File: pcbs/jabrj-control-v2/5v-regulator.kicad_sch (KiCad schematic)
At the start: 46 parts, among them Q401 DMN21D2UFB-7B, Q402 DMN21D2UFB-7B, Q403 DMN21D2UFB-7B, U401 AZV3001FZ4-7, U402 TPS259472ARPWR, U403 MAX20008AFOC/VY+T

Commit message: Layout almost done
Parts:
- D403, D404: footprint (none) -> project_footprints:C_0402
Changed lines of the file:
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@@
 			)
 		)
-		(property "Footprint" ""
+		(property "Footprint" "project_footprints:C_0402"
 			(at 228.6 109.22 90)
 			(hide yes)
@@
 			)
 		)
-		(property "Footprint" ""
+		(property "Footprint" "project_footprints:C_0402"
 			(at 254 109.22 90)
 			(hide yes)

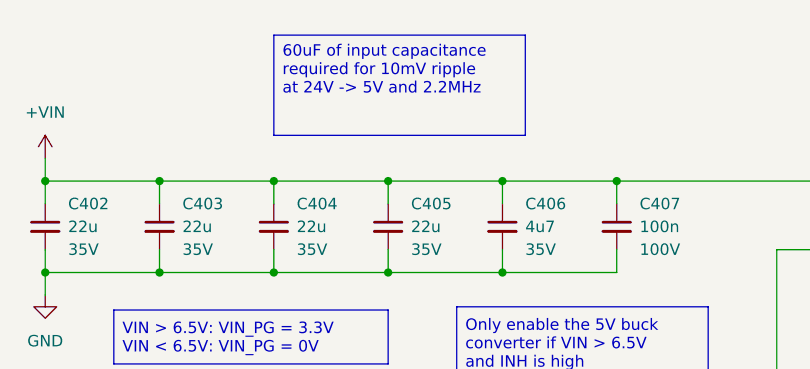
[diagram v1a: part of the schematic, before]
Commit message: 651 Unrouted
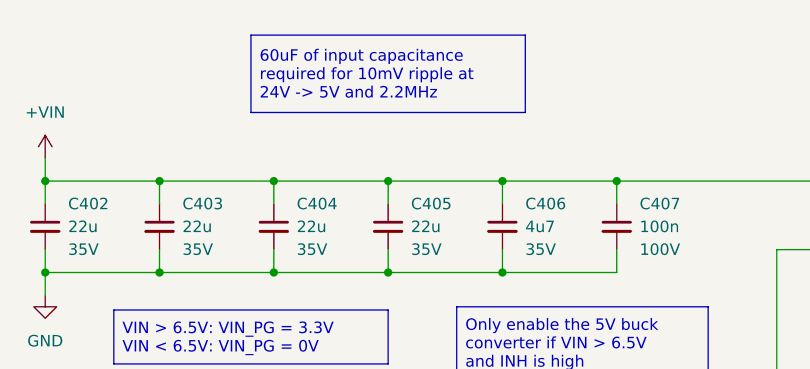
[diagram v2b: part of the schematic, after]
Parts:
- D403, D404: footprint project_footprints:C_0402 -> project_footprints:LED_0402
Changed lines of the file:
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@@
 	(text_box "60uF of input capacitance required for 10mV ripple at 24V -> 5V and 2.2MHz"
 		(exclude_from_sim no)
-		(at 76.2 32.0439 0)
-		(size 27.94 11.1361)
+		(at 73.66 32.044 0)
+		(size 30.48 8.596)
 		(margins 0.9525 0.9525 0.9525 0.9525)
 		(stroke
@@
 				(size 1.27 1.27)
 			)
-			(justify left top)
+			(justify left)
 		)
 	)
@@
 			)
 		)
-		(property "Footprint" "project_footprints:C_0402"
+		(property "Footprint" "project_footprints:LED_0402"
 			(at 228.6 109.22 90)
 			(hide yes)
@@
 			)
 		)
-		(property "Footprint" "project_footprints:C_0402"
+		(property "Footprint" "project_footprints:LED_0402"
 			(at 254 109.22 90)
 			(hide yes)
